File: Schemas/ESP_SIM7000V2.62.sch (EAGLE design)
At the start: 77 parts, among them J1 U.FL-R-SMT(01), J2 U.FL-R-SMT(01), J3 78646-3001, Q1 SI2305CDS, Q2 BSS138, Q3 SI2305CDS, Q4 BSS138, Q5 SI2305CDS, Q6 BSS138, Q7 BSS138, Q8 BSS138, Q9 BSS138, U1 ESP-WROOM-03, U2 TXB0108PWR, U4 MIC5239S, X1 S2B-PH-K-S, X2 B2B-PH-K-S

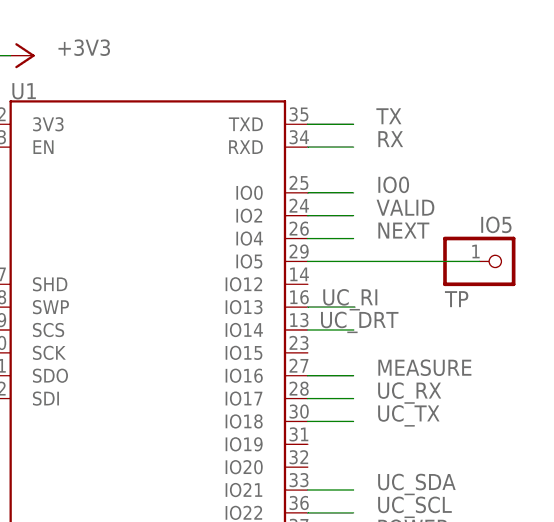
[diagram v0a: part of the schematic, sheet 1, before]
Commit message: Modifs EAGLE et Compte rendu
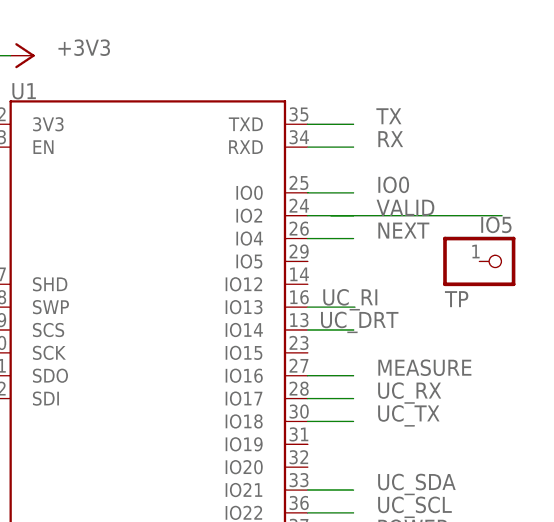
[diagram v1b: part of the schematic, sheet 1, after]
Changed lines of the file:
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@@
 <pinref part="U1" gate="G$1" pin="IO5"/>
 <pinref part="IO5" gate="G$1" pin="1"/>
-<wire x1="231.14" y1="147.32" x2="250.19" y2="147.32" width="0.1524" layer="91"/>
+<wire x1="233.68" y1="152.4" x2="252.73" y2="152.4" width="0.1524" layer="91"/>
 </segment>
 </net>
